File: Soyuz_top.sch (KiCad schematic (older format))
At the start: 46 parts, among them SW1 SW_Push, U1 ProMicro

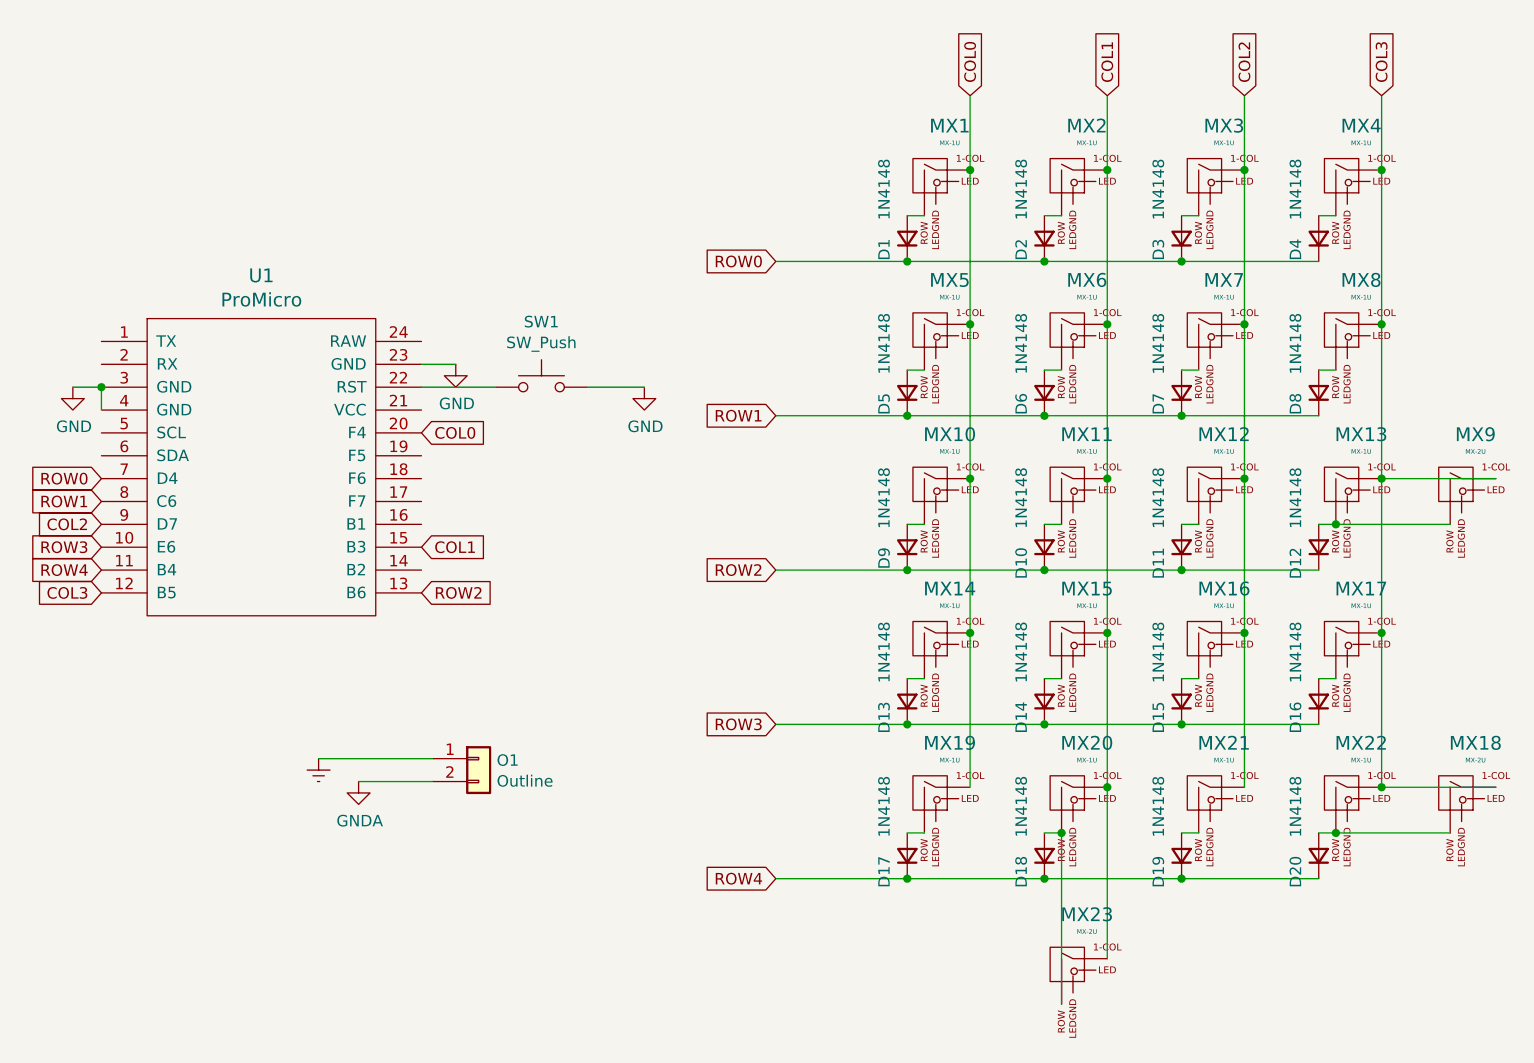
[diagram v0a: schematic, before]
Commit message: Updating outlines
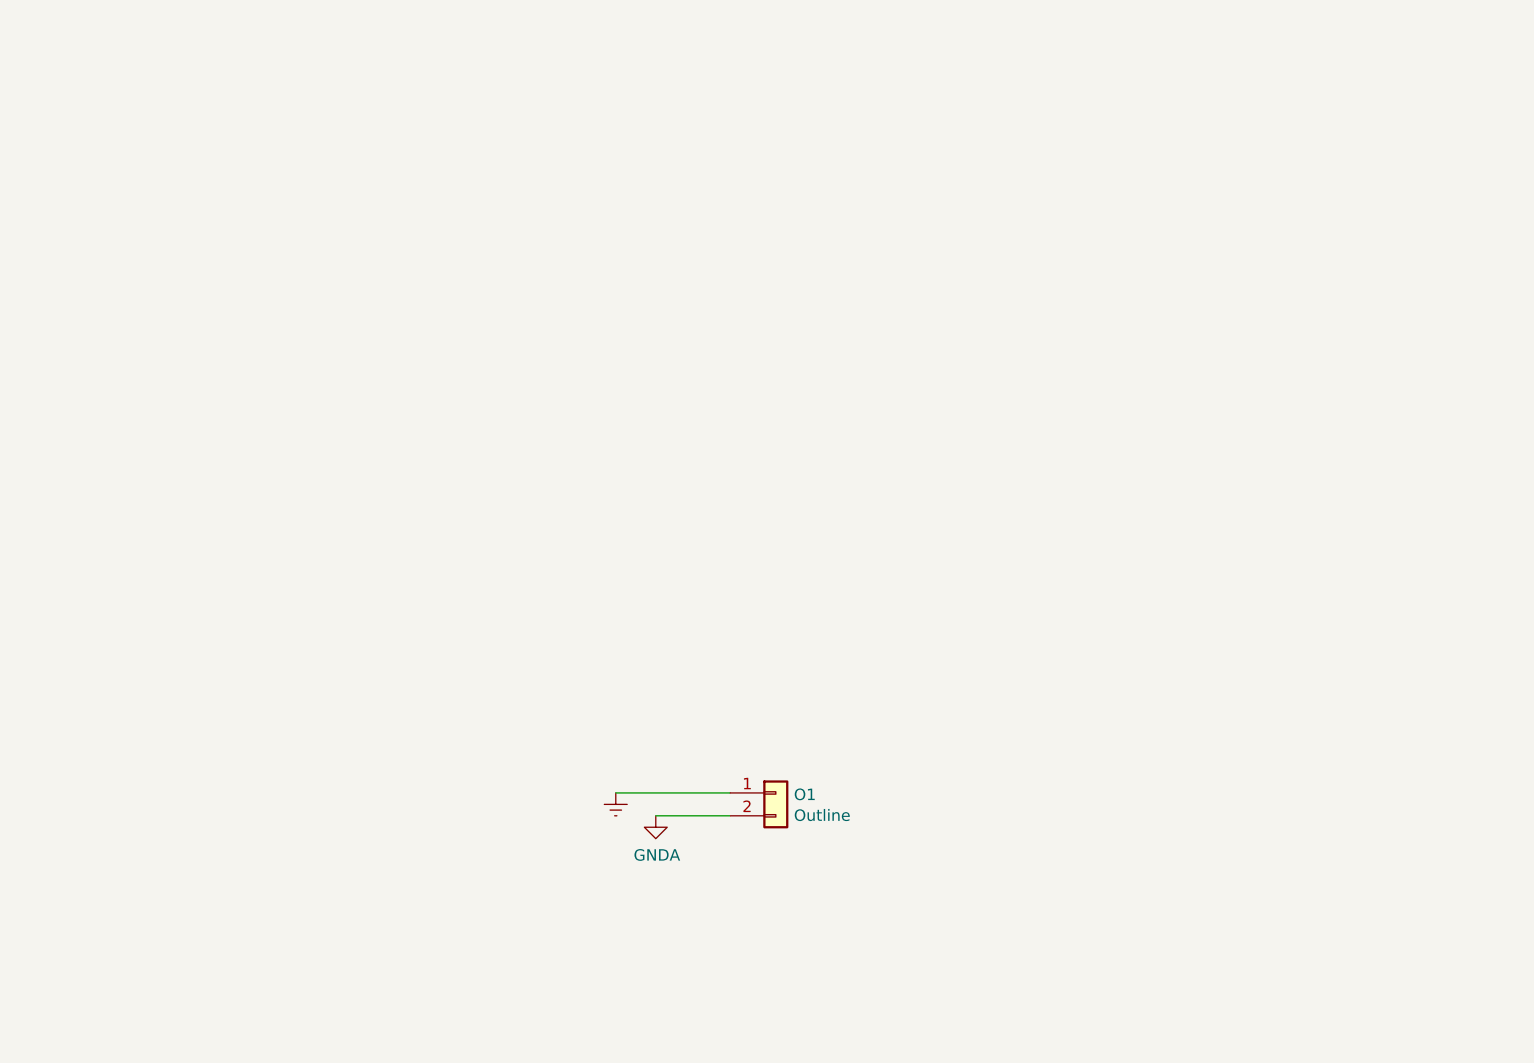
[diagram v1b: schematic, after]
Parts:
- removed D1, D10, D11, D12, D13, D14, D15, D16, D17, D18, D19, D2, D20, D3, D4, D5, D6, D7, D8, D9: 1N4148, Diodes_THT:D_DO-35_SOD27_P7.62mm_Horizontal, symbol Device:D_Small
- removed MX1, MX10, MX11, MX12, MX13, MX14, MX15, MX16, MX17, MX19, MX2, MX20, MX21, MX22, MX3, MX4, MX5, MX6, MX7, MX8: MX-1U, MX_Alps_Hybrid:MX-1U-NoLED, symbol MX_Alps_Hybrids:MX-1U
- removed MX18, MX23, MX9: MX-2U, MX_Alps_Hybrid:MX-2U-ReversedStabilizers-NoLED, symbol MX_Alps_Hybrids:MX-1U
- removed SW1: SW_Push, random-keyboard-parts:PushButton_6x6mm_TH_Pretty, symbol Switch:SW_Push
- removed U1: ProMicro, promicro:ProMicro-EnforcedTop, symbol promicro:ProMicro
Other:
- moved on the sheet: O1
